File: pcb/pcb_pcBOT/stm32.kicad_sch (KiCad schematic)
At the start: 16 parts, among them J301 ST_link, SW301 Reset_Button, U301 STM32G431KBT6, U302 LD3985M33R_SOT23

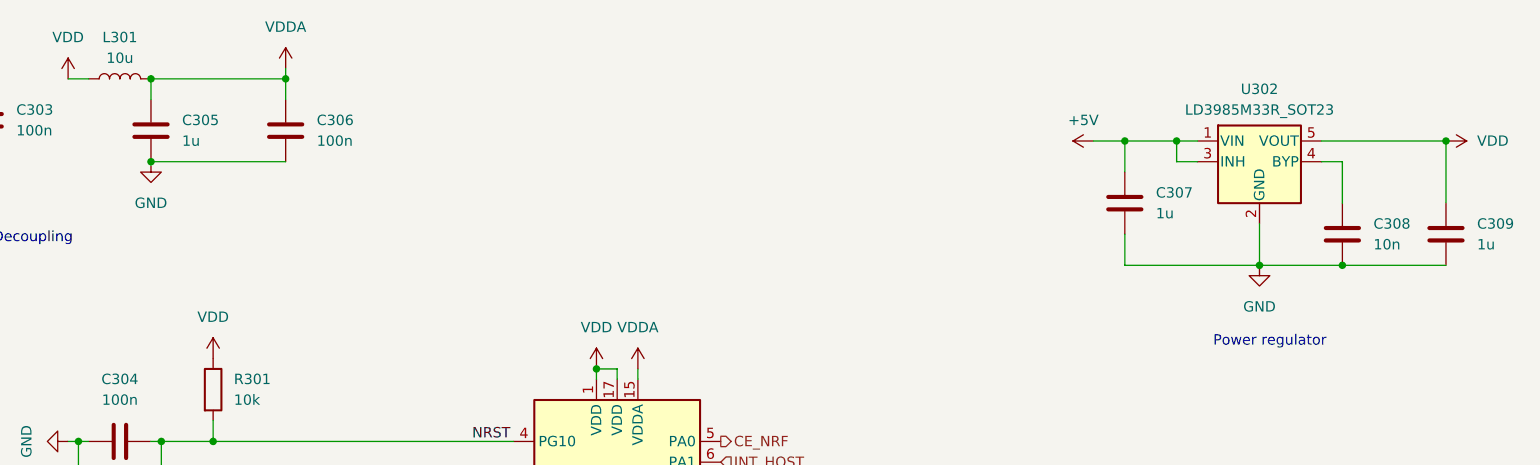
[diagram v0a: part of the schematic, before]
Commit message: Ajout empreintes (incomplet) + test erc correct
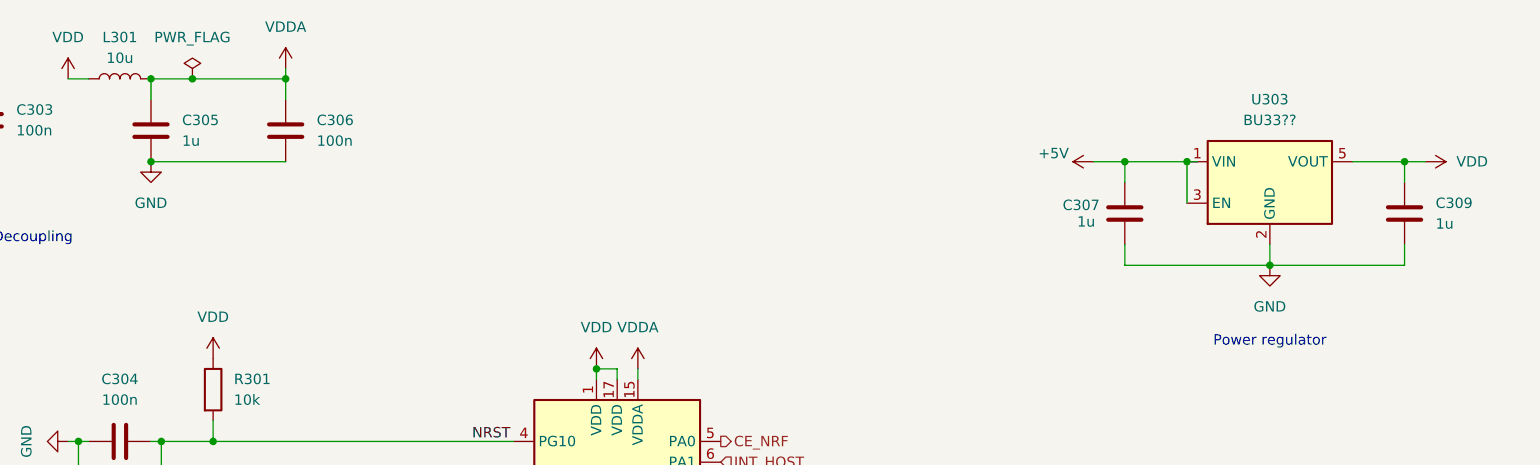
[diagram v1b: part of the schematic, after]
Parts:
- removed C308: 10n, symbol Device:C
- removed U302: LD3985M33R_SOT23, Package_TO_SOT_SMD:SOT-23-5, symbol Regulator_Linear:LD3985M33R_SOT23
- added U303: BU33??, Package_TO_SOT_SMD:TSOT-23-5, symbol Regulator_Linear:MIC5365-3.3YD5
- C301, C302, C303, C304, C305, C306, C307, C309: footprint (none) -> Capacitor_SMD:C_0805_2012Metric_Pad1.18x1.45mm_HandSolder
- J301: footprint (none) -> Connector_PinHeader_1.27mm:PinHeader_2x07_P1.27mm_Vertical_SMD
- L301: footprint (none) -> Inductor_SMD:L_0805_2012Metric_Pad1.05x1.20mm_HandSolder
- R301, R302: footprint (none) -> Resistor_SMD:R_0805_2012Metric_Pad1.20x1.40mm_HandSolder
- SW301: footprint (none) -> Button_Switch_THT:SW_PUSH_6mm
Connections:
- net +5V: now also U303.1 (VIN), U303.3 (EN)
- net GND: now also U303.2 (GND)
- net VDD: now also U303.5 (VOUT)
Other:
- moved on the sheet: C307, C309

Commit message: Revert "Ajout empreintes (incomplet) + test erc correct"
This reverts commit 267ed5519d67c336b99c9c80b0ac2067182b82a3.
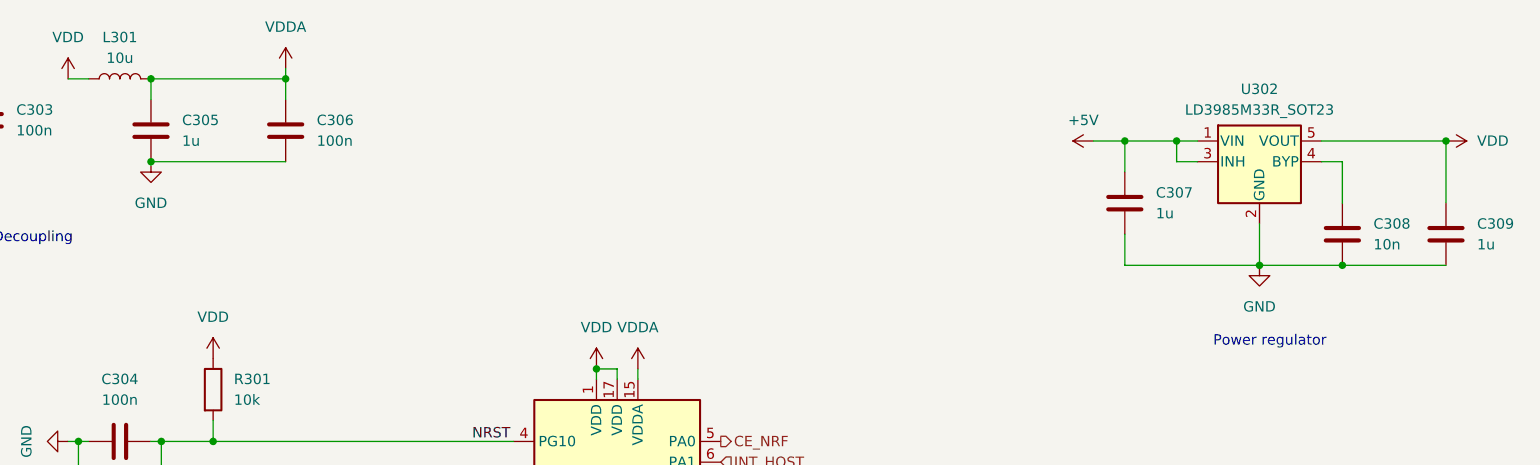
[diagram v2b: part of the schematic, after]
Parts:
- removed U303: BU33??, Package_TO_SOT_SMD:TSOT-23-5, symbol Regulator_Linear:MIC5365-3.3YD5
- added C308: 10n, symbol Device:C
- added U302: LD3985M33R_SOT23, Package_TO_SOT_SMD:SOT-23-5, symbol Regulator_Linear:LD3985M33R_SOT23
- C301, C302, C303, C304, C305, C306, C307, C309: footprint Capacitor_SMD:C_0805_2012Metric_Pad1.18x1.45mm_HandSolder -> (none)
- J301: footprint Connector_PinHeader_1.27mm:PinHeader_2x07_P1.27mm_Vertical_SMD -> (none)
- L301: footprint Inductor_SMD:L_0805_2012Metric_Pad1.05x1.20mm_HandSolder -> (none)
- R301, R302: footprint Resistor_SMD:R_0805_2012Metric_Pad1.20x1.40mm_HandSolder -> (none)
- SW301: footprint Button_Switch_THT:SW_PUSH_6mm -> (none)
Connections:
- net +5V: now also U302.1 (VIN), U302.3 (INH)
- net GND: now also C308.2, U302.2 (GND)
- net VDD: now also U302.5 (VOUT)
- new net: C308.1, U302.4 (BYP)
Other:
- moved on the sheet: C307, C309
